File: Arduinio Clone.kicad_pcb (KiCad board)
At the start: 2 copper layers, 50.8 x 25.4 mm, 17 parts, among them J1 Serial, J2 Digital Pins, J3 ICSP, J4 I2C, U1 DS1337_GM, U2 24LC1025, U3 ATmega328P-A, U4 24LC1025, Y1 Crystal 32MHz, Y2 Crystal 16MHz

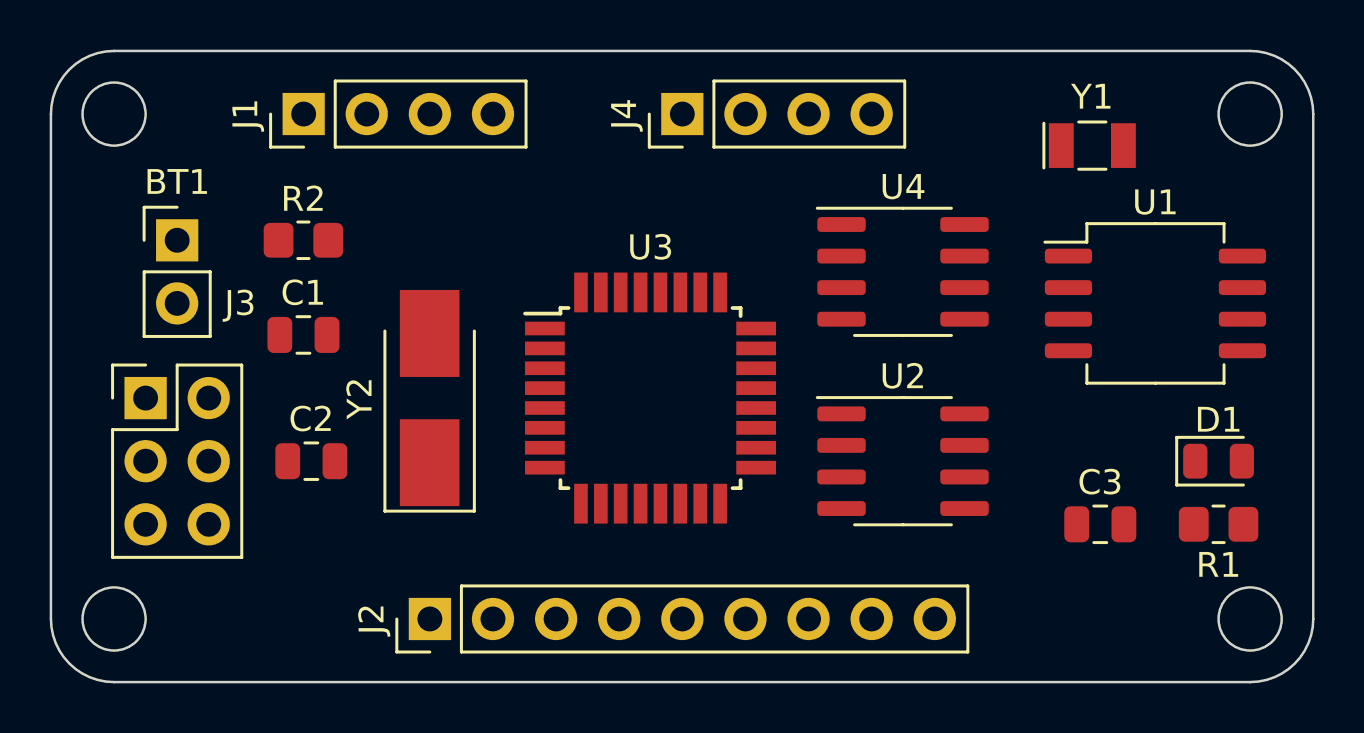
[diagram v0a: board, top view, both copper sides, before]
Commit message: Imported generated Spectra sessionfile and ran DRC
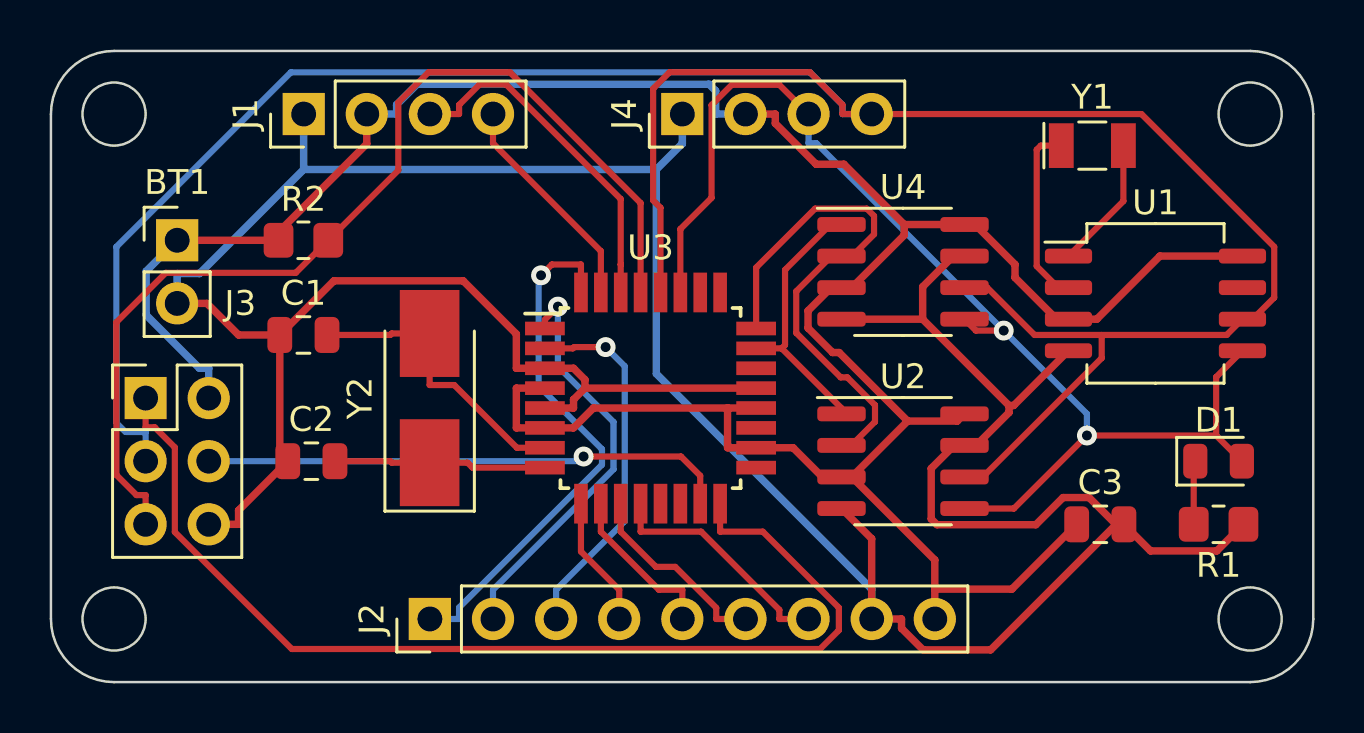
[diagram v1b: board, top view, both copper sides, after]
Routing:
- net GNDPWR: track 0.00 -> 141.7 mm
- net /VCC: track 0.00 -> 111.9 mm
- net /SCK: track 0.00 -> 104.9 mm
- net /SDA: track 0.00 -> 49.0 mm, vias 0 -> 2
- net /MISO: track 0.00 -> 43.2 mm
- net /RESET: track 0.00 -> 41.5 mm
- net /ADDR2: track 0.00 -> 21.6 mm
- net /D2: track 0.00 -> 21.4 mm, vias 0 -> 1
- net /MOSI: track 0.00 -> 21.3 mm, vias 0 -> 1
- net /D3: track 0.00 -> 16.6 mm, vias 0 -> 1
- net /D4: track 0.00 -> 14.9 mm, vias 0 -> 1
- net /RX: track 0.00 -> 14.1 mm
- net Net-(C1-Pad2): track 0.00 -> 11.9 mm
- net /ADDR1: track 0.00 -> 10.9 mm
- net /D8: track 0.00 -> 9.56 mm
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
